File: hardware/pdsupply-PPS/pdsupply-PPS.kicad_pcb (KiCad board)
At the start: 2 copper layers, 70 x 50 mm, 74 parts, among them IC1 LTM8083EY#PBF, IC2 FPF2895UCX, J1 USB4505-03-0-A_REVA, J2 USB4505-03-0-A_REVA, J3 Screw_Terminal_01x02, U1 FUSB307BMPX, U2 ADUM3160, U3 ACS71240KEXBLT-050U5, U4 STM32L432KCUx

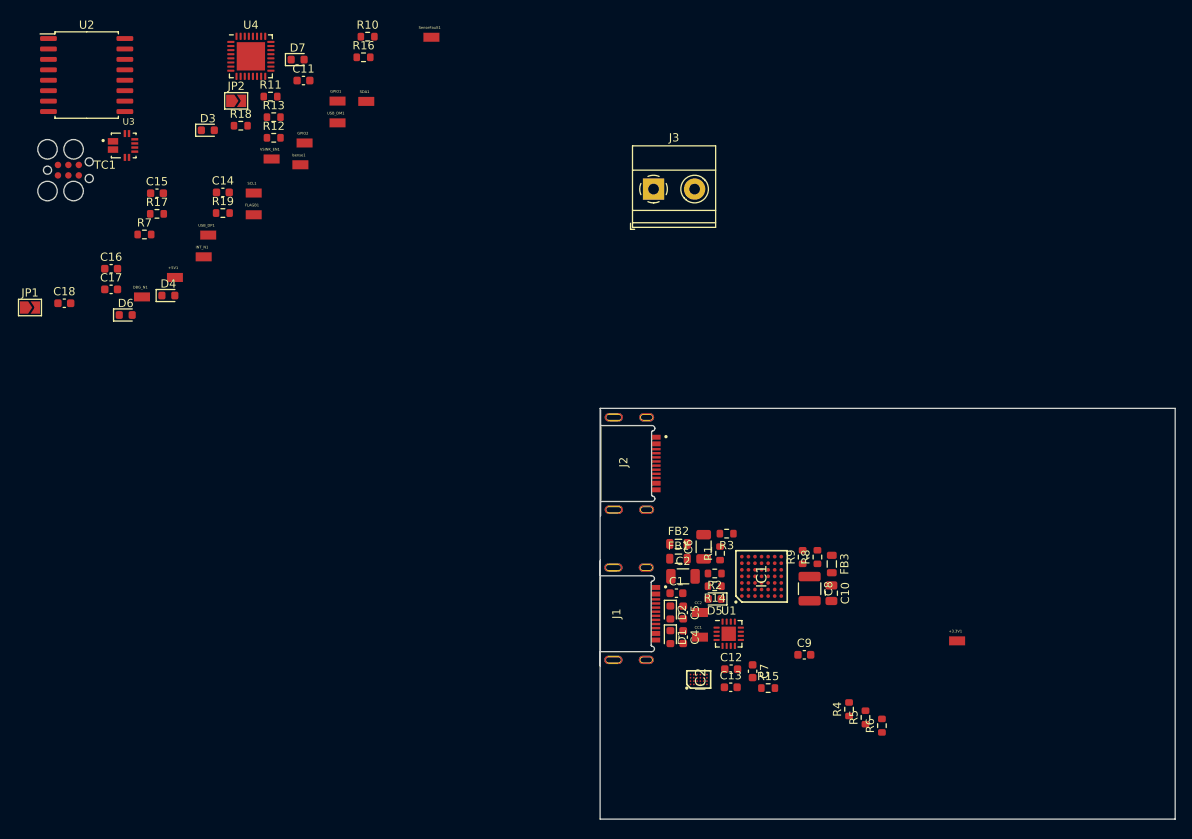
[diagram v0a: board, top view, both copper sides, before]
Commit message: component placement done
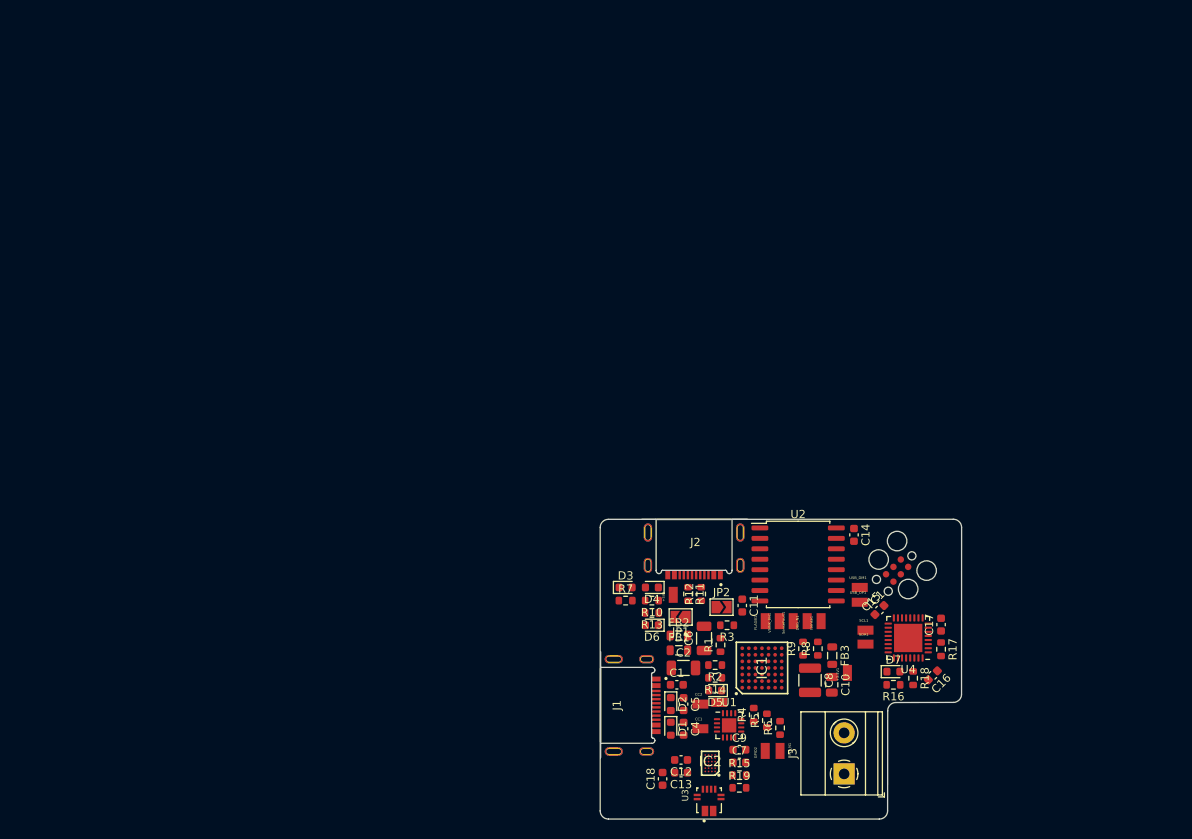
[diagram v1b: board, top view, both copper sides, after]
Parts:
- moved TC1 112.0 mm to (146.2, 89.7), turned to -135 degrees
- moved C16 111.6 mm to (150.5, 102.5), turned to -135 degrees
- moved R17 109.2 mm to (151.5, 99.3), turned to -90 degrees
- moved C17 109.0 mm to (151.5, 96.3), turned to 90 degrees
- moved U3 106.9 mm to (123.3, 117.7), turned to 90 degrees
- moved U4 106.8 mm to (147.5, 98.0), turned to 180 degrees
- moved R18 105.9 mm to (148.1, 102.8), turned to -90 degrees
- moved U2 105.1 mm to (134.1, 89.0)
- moved D7 104.0 mm to (145.7, 102.0)
- moved C15 101.5 mm to (144.0, 94.5), turned to 45 degrees
- moved R16 100.0 mm to (145.7, 103.7), turned to 180 degrees
- moved R19 94.1 mm to (127.0, 116.2)
- moved C18 93.0 mm to (117.6, 115.1), turned to 90 degrees
- moved GPIO2 92.9 mm to (130.1, 111.7), turned to 90 degrees
- moved INT_N1 92.4 mm to (131.9, 111.7), turned to -90 degrees
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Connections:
- J3 pad 1: GND -> Net-(J3-Pad1)
- J3 pad 2: Net-(J3-Pad2) -> GND
- U3 pad 3: Net-(J3-Pad2) -> Net-(J3-Pad1)
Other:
- board size 70 x 50 mm -> 44 x 36.5 mm
